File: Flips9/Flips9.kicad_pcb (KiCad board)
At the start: 2 copper layers, 100 x 100 mm, 45 parts, among them CN1 UFP2810, U1 74238, U11 74238, U12 74238, U13 TD62783, U14 ULN2803/2003, U21 74238, U22 74238, U23 TD62783, U24 ULN2803/2003, U31 74238, U32 74238, U33 TD62783, U34 ULN2803/2003

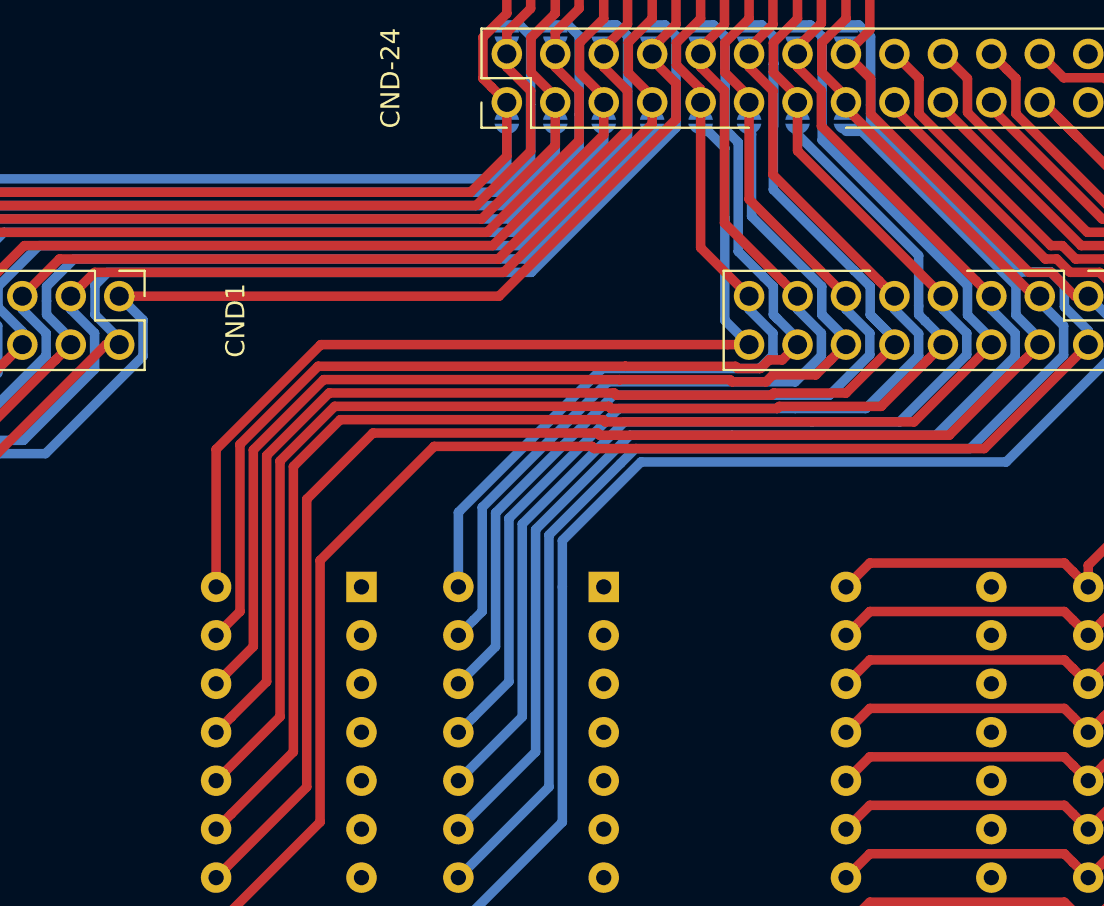
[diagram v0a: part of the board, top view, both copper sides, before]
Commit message: improve traces
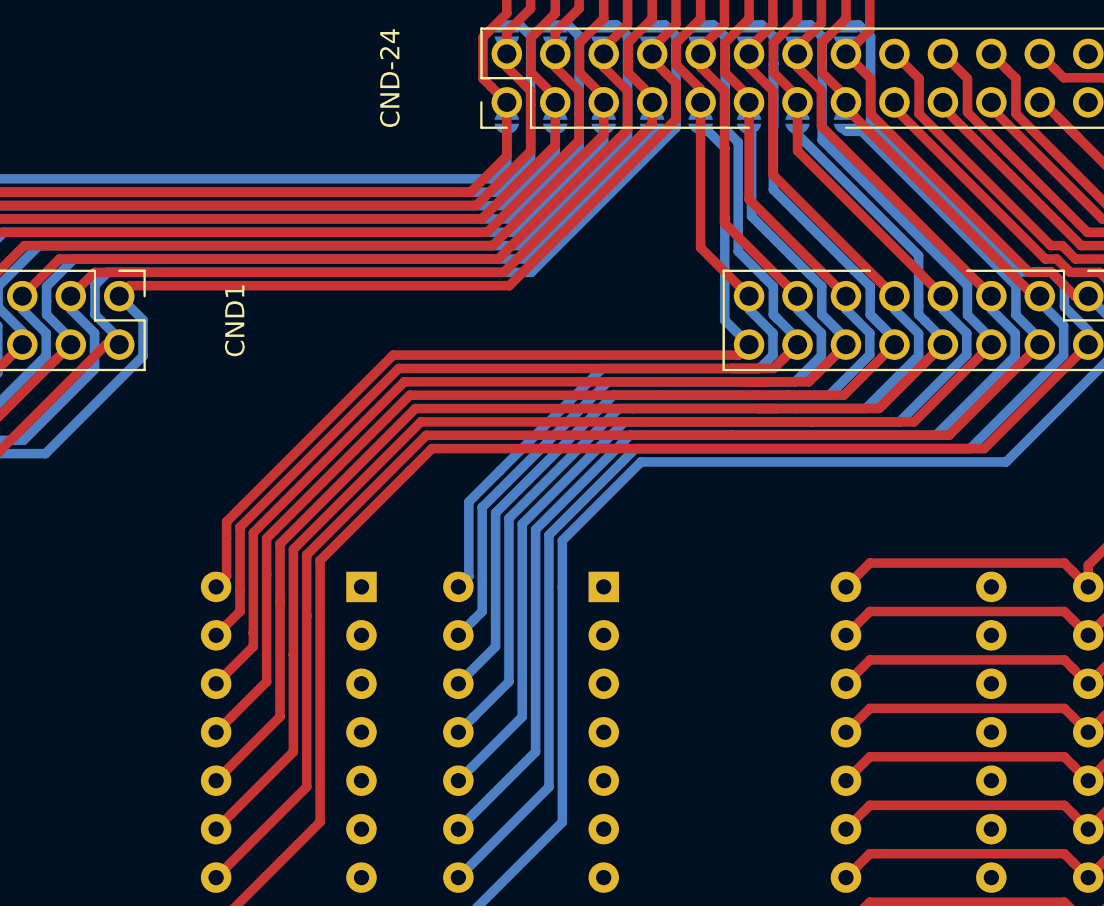
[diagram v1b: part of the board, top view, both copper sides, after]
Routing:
- net /SX13: track 69.9 -> 72.8 mm
- net /SX12: track 76.7 -> 74.1 mm
- net /SX14: track 81.4 -> 78.7 mm
- net /SX9: track 49.9 -> 47.4 mm
- net /SX15: track 79.6 -> 77.8 mm
- net /SX11: track 61.9 -> 62.8 mm
